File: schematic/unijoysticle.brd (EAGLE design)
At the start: 70.8 x 66 mm, 8 parts, among them CN1 External Battery, IC1 4066N, IC2 4066N, IC3 4066N, X1 Joy #1, X2 Joy #2

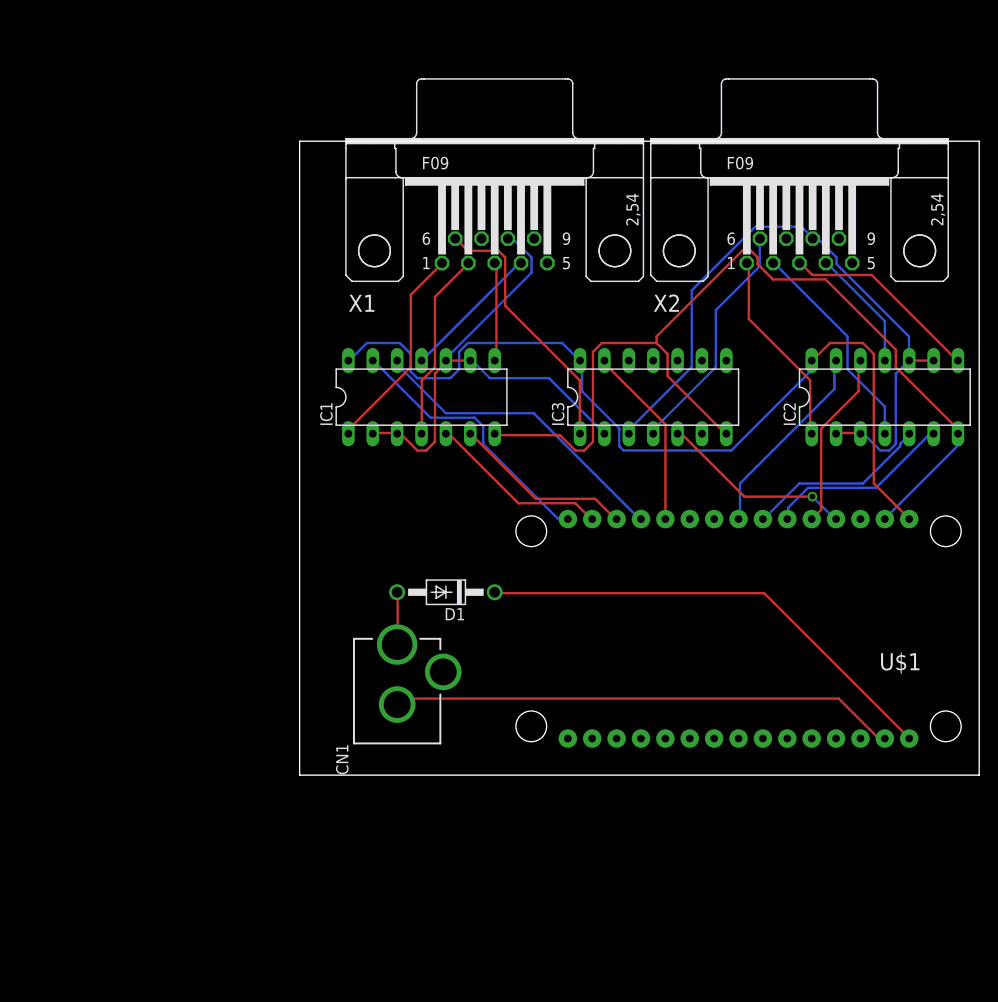
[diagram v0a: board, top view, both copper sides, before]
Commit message: fix: schematic & board fixed
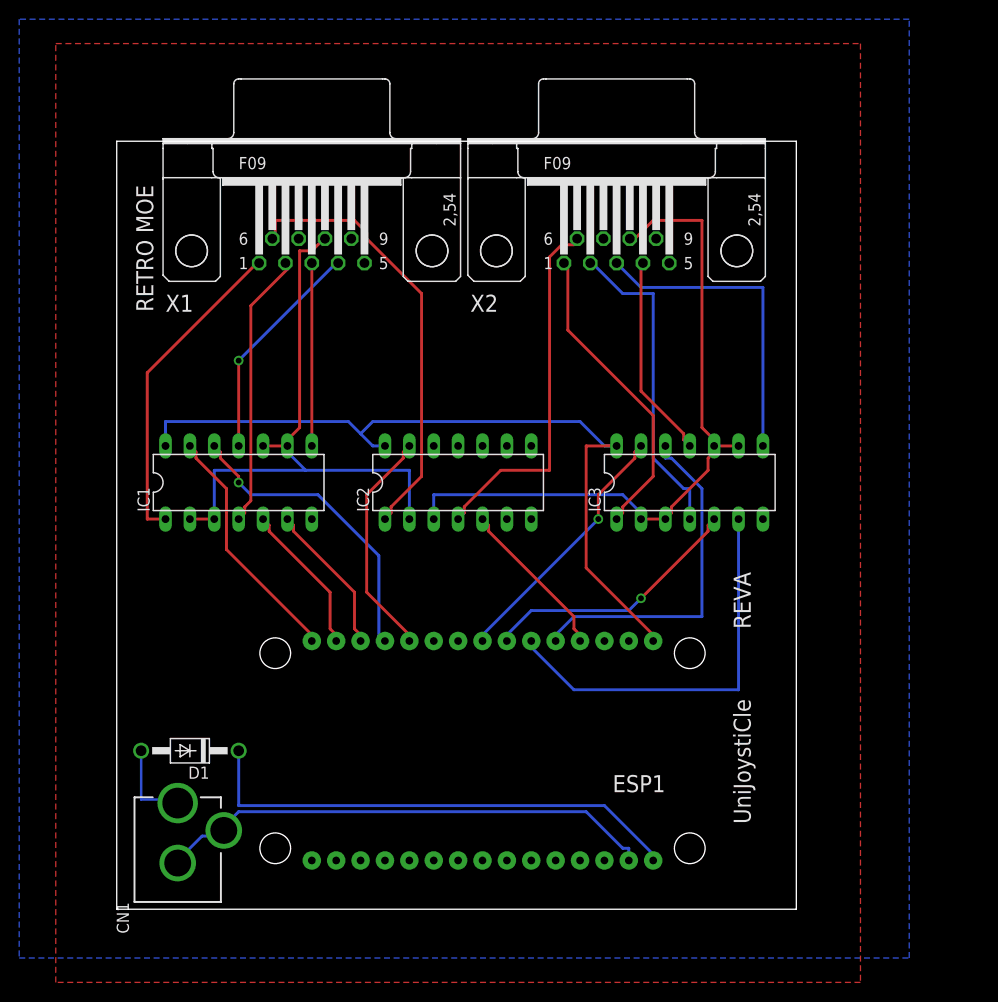
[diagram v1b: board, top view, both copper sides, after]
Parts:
- removed U$1: ESP12E_DEVKIT, ESP12E_DEVKIT:ESP12E_DEVKIT
- added ESP1: ESP12E_DEVKIT, ESP12E_DEVKIT:ESP12E_DEVKIT
- CN1: value External Battery -> 3.3V - 9V
- moved IC2 45.3 mm to (35.6, 44.5)
- moved D1 31.4 mm to (7.62, 16.5)
- moved CN1 28.2 mm to (6.35, -2.54)
- moved IC1 21.0 mm to (12.7, 44.5)
- moved X2 19.1 mm to (52.1, 68.6)
- moved X1 19.0 mm to (20.3, 68.6)
- moved IC3 9.67 mm to (59.7, 44.5)
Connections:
- removed net GNDBREAK: CN1.GNDBREAK
- removed net N$24: D1.C, U$1.VIN
- removed net N$25: CN1.GND, U$1.GND@1
- new net 3.3V: CN1.GND, CN1.GNDBREAK, ESP1.GND@1
- new net 5V: D1.C, ESP1.VIN
- net GND: now also ESP1.GND@3; no longer U$1.GND@3
- net N$1: now also ESP1.D0; no longer U$1.D0
- net N$13: now also IC3.1; no longer IC2.1
- net N$14: now also IC3.4; no longer IC2.4
- net N$15: now also IC3.8; no longer IC2.8
- net N$16: now also IC3.11; no longer IC2.11
- net N$17: now also IC2.2; no longer IC3.2
- net N$18: now also IC3.10, IC3.2, IC3.9; no longer IC2.10, IC2.2, IC2.9
- net N$19: now also ESP1.D4, IC2.13; no longer IC3.13, U$1.D4
- net N$2: now also ESP1.D1; no longer U$1.D1
- net N$20: now also ESP1.RX, IC2.5; no longer IC3.5, U$1.RX
- net N$21: now also IC2.1; no longer IC3.1
- net N$22: now also IC2.4; no longer IC3.4
- net N$3: now also ESP1.D2; no longer U$1.D2
- net N$4: now also ESP1.D3; no longer U$1.D3
- net N$5: now also ESP1.D5, IC3.13; no longer IC2.13, U$1.D5
- net N$6: now also ESP1.D6, IC3.5; no longer IC2.5, U$1.D6
- net N$7: now also ESP1.D7, IC3.6; no longer IC2.6, U$1.D7
- net N$8: now also ESP1.D8, IC3.12; no longer IC2.12, U$1.D8
- net VCC: now also ESP1.3V3@2; no longer U$1.3V3@2
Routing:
- net GND: track 97.7 -> 0.00 mm
- net 3.3V: track 0.00 -> 53.0 mm
- net N$25: track 52.9 -> 0.00 mm
- net 5V: track 0.00 -> 51.6 mm
- net N$24: track 49.5 -> 0.00 mm
- net N$7: track 19.6 -> 41.8 mm
- net N$21: track 27.6 -> 46.1 mm
- net N$8: track 18.7 -> 36.4 mm
- net N$22: track 24.9 -> 38.3 mm
- net N$15: track 20.7 -> 32.8 mm
- net N$9: track 21.8 -> 33.5 mm
- net N$13: track 20.7 -> 32.3 mm
- net VCC: track 92.8 -> 81.1 mm
- net N$14: track 22.6 -> 33.3 mm
- net N$10: track 19.8 -> 29.0 mm
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- added copper zone on layer 1, net GND
- added copper zone on layer 16, net GND
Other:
- board size 70.8 x 66 mm -> 70.8 x 80 mm
- board text added: "RETRO MOE"
- board text added: "REVA"
- board text added: "UniJoystiCle"

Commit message: fix: board fixes
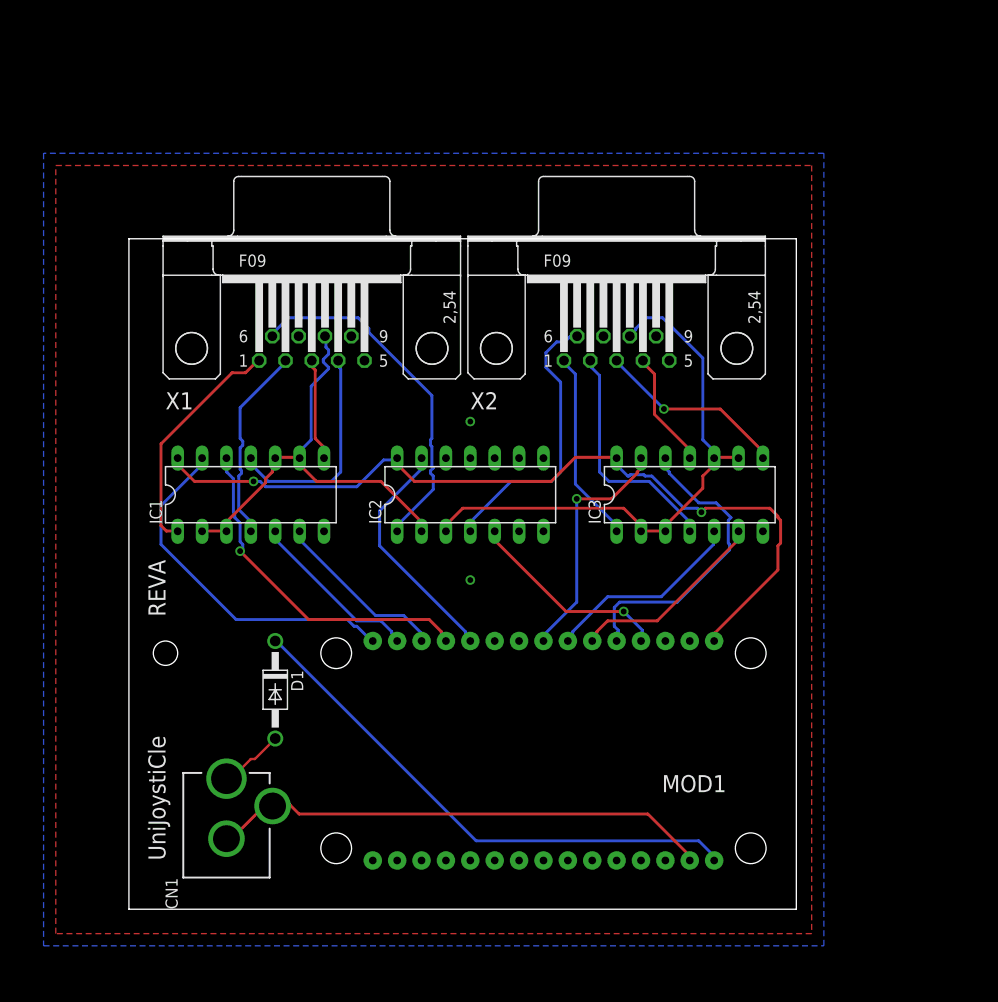
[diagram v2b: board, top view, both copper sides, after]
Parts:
- removed ESP1: ESP12E_DEVKIT, ESP12E_DEVKIT:ESP12E_DEVKIT
- added MOD1: NodeMCU Amica v1.0, ESP12E_DEVKIT:ESP12E_DEVKIT
- CN1: value 3.3V - 9V -> DC JACK
- D1: value 1N4004 -> 1N4001
- X1: value Joy #1 -> DSUB 9
- X2: value Joy #2 -> DSUB 9
- moved D1 10.9 mm to (16.5, 22.9), turned to 270 degrees
- moved X1 10.2 mm to (20.3, 58.4)
- moved X2 10.2 mm to (52.1, 58.4)
- moved CN1 5.68 mm to (11.4, 0.00)
- moved IC1 1.80 mm to (14.0, 43.2)
- moved IC2 1.80 mm to (36.8, 43.2)
- moved IC3 1.27 mm to (59.7, 43.2)
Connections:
- net 3.3V: now also MOD1.GND@1; no longer ESP1.GND@1
- net 5V: now also MOD1.VIN; no longer ESP1.VIN
- net GND: now also MOD1.GND@3; no longer ESP1.GND@3
- net N$1: now also MOD1.D0; no longer ESP1.D0
- net N$19: now also MOD1.D4; no longer ESP1.D4
- net N$2: now also MOD1.D1; no longer ESP1.D1
- net N$20: now also MOD1.RX; no longer ESP1.RX
- net N$3: now also MOD1.D2; no longer ESP1.D2
- net N$4: now also MOD1.D3; no longer ESP1.D3
- net N$5: now also MOD1.D5; no longer ESP1.D5
- net N$6: now also MOD1.D6; no longer ESP1.D6
- net N$7: now also MOD1.D7; no longer ESP1.D7
- net N$8: now also MOD1.D8; no longer ESP1.D8
- net VCC: now also MOD1.3V3@2; no longer ESP1.3V3@2
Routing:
- net N$7: track 41.8 -> 20.8 mm
- net N$17: track 62.9 -> 46.4 mm
- net N$18: track 72.7 -> 59.2 mm
- net N$15: track 32.8 -> 20.0 mm, vias 0 -> 1
- net N$13: track 32.3 -> 20.1 mm
- net N$1: track 25.6 -> 37.0 mm
- net N$16: track 21.4 -> 12.2 mm
- net N$9: track 33.5 -> 24.5 mm
- net N$21: track 46.1 -> 37.3 mm
- net N$14: track 33.3 -> 24.6 mm
- net N$22: track 38.3 -> 29.6 mm
- net N$11: track 19.1 -> 10.7 mm
- net N$10: track 29.0 -> 20.7 mm
- net N$6: track 27.6 -> 21.1 mm, vias 1 -> 0
- net VCC: track 81.1 -> 87.3 mm, vias 0 -> 2
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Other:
- board size 70.8 x 80 mm -> 69.5 x 69.8 mm
- board text removed: "RETRO MOE"
